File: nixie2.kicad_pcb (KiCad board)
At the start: 2 copper layers, 68.5 x 181 mm, 50 parts, among them J1 AVR-ISP-6, J14 Conn_01x10_Female, SW1 Conn_01x02_Male, SW2 Conn_01x02_Male, SW3 Conn_01x02_Male, SW4 Conn_01x02_Male, SW5 Conn_01x02_Male, SW6 Conn_01x02_Male, U1 ATmega8-16PU, U10 74141, U11 L7805, U2 74HC595, U3 74HC595, U4 74HC595, U5 74141, U6 74141, U7 74141, U8 74141, U9 74141, X1 CXO_DIP8

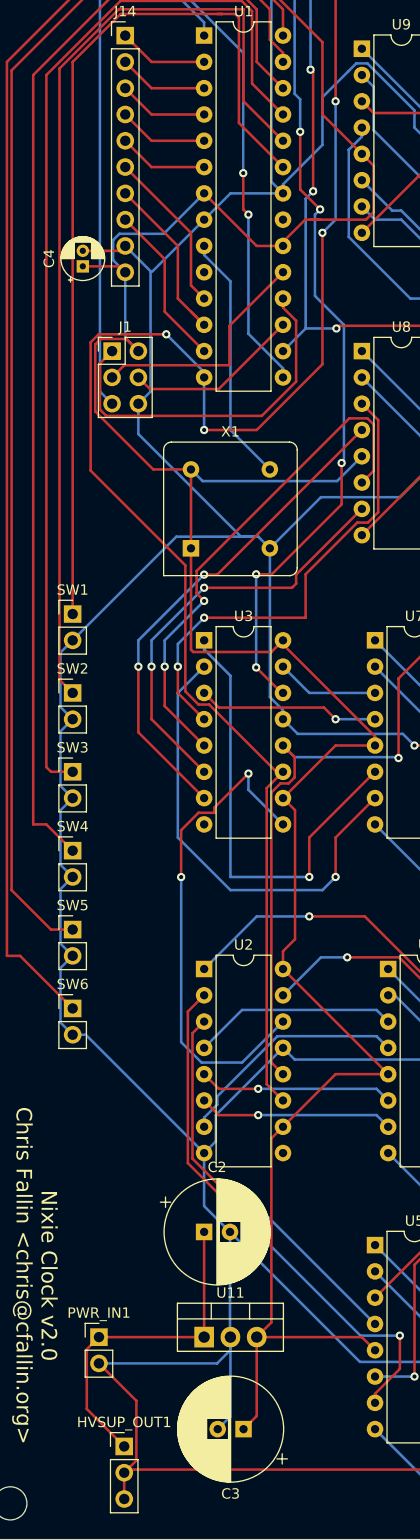
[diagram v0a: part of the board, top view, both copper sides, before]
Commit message: Update.
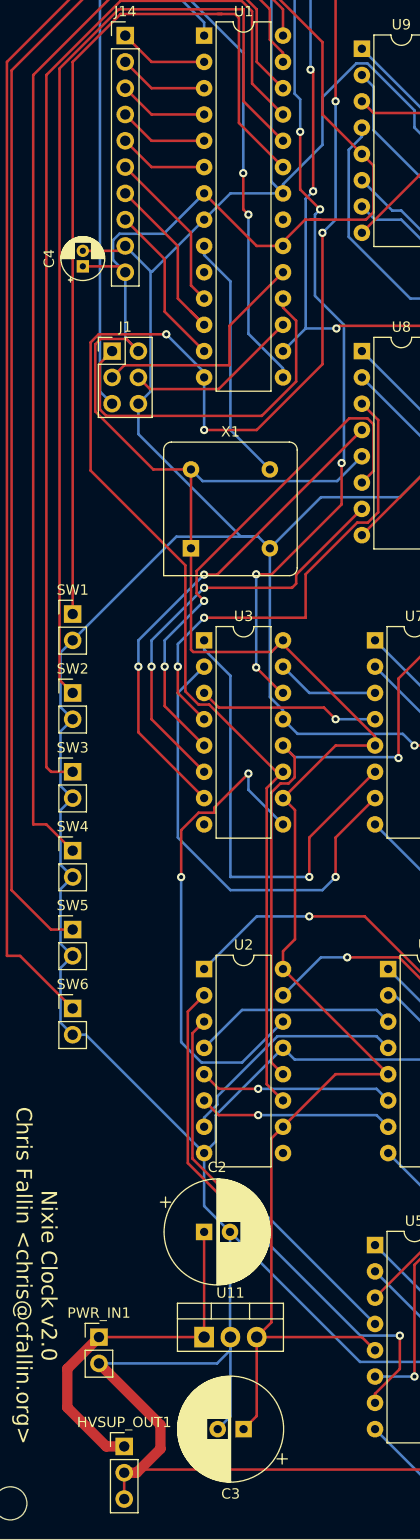
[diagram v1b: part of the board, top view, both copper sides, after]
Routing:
- net GND: track 461.4 -> 464.1 mm
- net Net-(C2-Pad1): track 32.9 -> 35.4 mm
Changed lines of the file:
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@@
     (thickness 1.6)
     (drawings 11)
-    (tracks 781)
+    (tracks 782)
     (zones 0)
     (modules 50)
@@
   )
   (setup
-    (last_trace_width 0.25)
+    (last_trace_width 1)
+    (user_trace_width 1)
     (trace_clearance 0.2)
     (zone_clearance 0.508)
@@
   (segment (start 89.734999 69.975001) (end 97.26 62.45) (width 0.25) (layer B.Cu) (net 4))
   (segment (start 89.545001 69.975001) (end 89.734999 69.975001) (width 0.25) (layer B.Cu) (net 4))
-  (segment (start 108.657499 50.657499) (end 106.15 53.164998) (width 0.25) (layer B.Cu) (net 4))
-  (segment (start 109.419999 49.894999) (end 108.657499 50.657499) (width 0.25) (layer B.Cu) (net 4))
-  (segment (start 86.63 68) (end 87.1 67.53) (width 0.25) (layer F.Cu) (net 4))
-  (segment (start 83 68) (end 86.63 68) (width 0.25) (layer F.Cu) (net 4))
-  (segment (start 88.175001 179.095001) (end 84.56 175.48) (width 0.25) (layer F.Cu) (net 4))
-  (segment (start 88.175001 184.864999) (end 88.175001 179.095001) (width 0.25) (layer F.Cu) (net 4))
-  (segment (start 87 186.04) (end 88.175001 184.864999) (width 0.25) (layer F.Cu) (net 4))
-  (segment (start 87 188.58) (end 87 186.04) (width 0.25) (layer F.Cu) (net 4))
-  (segment (start 87.305001 185.734999) (end 87 186.04) (width 0.25) (layer F.Cu) (net 4))
-  (segment (start 129.507082 185.734999) (end 87.305001 185.734999) (width 0.25) (layer F.Cu) (net 4))
+  (segment (start 109.419999 49.894999) (end 106.15 53.164998) (width 0.25) (layer B.Cu) (net 4))
+  (segment (start 86.63 68) (end 87.1 67.53) (width 0.25) (layer F.Cu) (net 4) (status 30))
+  (segment (start 83 68) (end 86.63 68) (width 0.25) (layer F.Cu) (net 4) (status 30))
+  (segment (start 87 188.58) (end 87 186.04) (width 0.25) (layer F.Cu) (net 4) (status 30))
+  (segment (start 87.305001 185.734999) (end 87 186.04) (width 0.25) (layer F.Cu) (net 4) (status 30))
+  (segment (start 129.507082 185.734999) (end 87.305001 185.734999) (width 0.25) (layer F.Cu) (net 4) (status 20))
   (segment (start 135 180.242081) (end 129.507082 185.734999) (width 0.25) (layer F.Cu) (net 4))
-  (segment (start 135 179.04) (end 135 180.242081) (width 0.25) (layer F.Cu) (net 4))
+  (segment (start 135 179.04) (end 135 180.242081) (width 0.25) (layer F.Cu) (net 4) (status 10))
+  (segment (start 88.202081 186.04) (end 90.5 183.742081) (width 1) (layer F.Cu) (net 4))
+  (segment (start 87 186.04) (end 88.202081 186.04) (width 1) (layer F.Cu) (net 4) (status 10))
+  (segment (start 90.5 181.42) (end 84.56 175.48) (width 1) (layer F.Cu) (net 4) (status 20))
+  (segment (start 90.5 183.742081) (end 90.5 181.42) (width 1) (layer F.Cu) (net 4))
   (segment (start 94.575001 90.245001) (end 93.45 89.12) (width 0.25) (layer B.Cu) (net 6) (status 20))
   (segment (start 107.564999 90.245001) (end 94.575001 90.245001) (width 0.25) (layer B.Cu) (net 6))
@@
   (segment (start 105.01 64.99) (end 110.355002 64.99) (width 0.25) (layer F.Cu) (net 6))
   (segment (start 104.484998 64.99) (end 105.01 64.99) (width 0.25) (layer F.Cu) (net 6))
-  (segment (start 86.53 69.5) (end 87.1 70.07) (width 0.25) (layer F.Cu) (net 6))
-  (segment (start 83 69.5) (end 86.53 69.5) (width 0.25) (layer F.Cu) (net 6))
+  (segment (start 86.53 69.5) (end 87.1 70.07) (width 0.25) (layer F.Cu) (net 6) (status 30))
+  (segment (start 83 69.5) (end 86.53 69.5) (width 0.25) (layer F.Cu) (net 6) (status 30))
   (segment (start 87.005001 79.054999) (end 97.165001 79.054999) (width 0.25) (layer F.Cu) (net 7))
   (segment (start 85.83 80.23) (end 87.005001 79.054999) (width 0.25) (layer F.Cu) (net 7) (status 10))
@@
   (segment (start 84.56 172.94) (end 94.72 172.94) (width 0.25) (layer F.Cu) (net 13) (status 30))
   (segment (start 94.72 172.94) (end 94.72 162.78) (width 0.25) (layer F.Cu) (net 13) (status 30))
-  (segment (start 83.384999 174.115001) (end 84.56 172.94) (width 0.25) (layer F.Cu) (net 13))
-  (segment (start 83.384999 179.884999) (end 83.384999 174.115001) (width 0.25) (layer F.Cu) (net 13))
-  (segment (start 87 183.5) (end 83.384999 179.884999) (width 0.25) (layer F.Cu) (net 13))
+  (segment (start 84.56 172.94) (end 81.5 176) (width 1) (layer F.Cu) (net 13) (status 10))
+  (segment (start 85.266 183.5) (end 87 183.5) (width 1) (layer F.Cu) (net 13) (status 20))
+  (segment (start 81.5 179.734) (end 85.266 183.5) (width 1) (layer F.Cu) (net 13))
+  (segment (start 81.5 176) (end 81.5 179.734) (width 1) (layer F.Cu) (net 13))
   (segment (start 87.1 64.99) (end 90.91 68.8) (width 0.25) (layer F.Cu) (net 14) (status 10))
   (segment (start 90.91 73.88) (end 94.72 77.69) (width 0.25) (layer F.Cu) (net 14) (status 20))
@@
   (segment (start 112.895002 64.115002) (end 109.96 61.18) (width 0.25) (layer B.Cu) (net 115) (status 20))
   (segment (start 113.77 64.115002) (end 112.895002 64.115002) (width 0.25) (layer B.Cu) (net 115))
-  (segment (start 134.5 168) (end 134.5 164) (width 0.25) (layer B.Cu) (net 116))
-  (segment (start 134 140) (end 134.5 140.5) (width 0.25) (layer B.Cu) (net 117))
-  (segment (start 134 135) (end 134 140) (width 0.25) (layer B.Cu) (net 117))
-  (segment (start 135.5 112.5) (end 135.5 105.5) (width 0.25) (layer B.Cu) (net 118))
-  (segment (start 135.5 84.5) (end 135.5 76.5) (width 0.25) (layer B.Cu) (net 119))
-  (segment (start 135 53) (end 135 47) (width 0.25) (layer B.Cu) (net 120))
-  (segment (start 135 30.5) (end 135 23) (width 0.25) (layer B.Cu) (net 121))
-  (segment (start 138.14999 58.68999) (end 135 55.54) (width 0.25) (layer B.Cu) (net 122))
+  (segment (start 134.5 168) (end 134.5 164) (width 0.25) (layer B.Cu) (net 116) (status 30))
+  (segment (start 134 140) (end 134.5 140.5) (width 0.25) (layer B.Cu) (net 117) (status 30))
+  (segment (start 134 135) (end 134 140) (width 0.25) (layer B.Cu) (net 117) (status 30))
+  (segment (start 135.5 112.5) (end 135.5 105.5) (width 0.25) (layer B.Cu) (net 118) (status 30))
+  (segment (start 135.5 84.5) (end 135.5 76.5) (width 0.25) (layer B.Cu) (net 119) (status 30))
+  (segment (start 135 53) (end 135 47) (width 0.25) (layer B.Cu) (net 120) (status 30))
+  (segment (start 135 30.5) (end 135 23) (width 0.25) (layer B.Cu) (net 121) (status 30))
+  (segment (start 138.14999 58.68999) (end 135 55.54) (width 0.25) (layer B.Cu) (net 122) (status 20))
   (segment (start 138.14999 84.39001) (end 138.14999 58.68999) (width 0.25) (layer B.Cu) (net 122))
-  (segment (start 135.5 87.04) (end 138.14999 84.39001) (width 0.25) (layer B.Cu) (net 122))
-  (segment (start 135 55.54) (end 137.5 53.04) (width 0.25) (layer B.Cu) (net 122))
-  (segment (start 137.5 35.54) (end 135 33.04) (width 0.25) (layer B.Cu) (net 122))
+  (segment (start 135.5 87.04) (end 138.14999 84.39001) (width 0.25) (layer B.Cu) (net 122) (status 10))
+  (segment (start 135 55.54) (end 137.5 53.04) (width 0.25) (layer B.Cu) (net 122) (status 10))
+  (segment (start 137.5 35.54) (end 135 33.04) (width 0.25) (layer B.Cu) (net 122) (status 20))
   (segment (start 137.5 53.04) (end 137.5 35.54) (width 0.25) (layer B.Cu) (net 122))
-  (segment (start 138.14999 112.39001) (end 135.5 115.04) (width 0.25) (layer B.Cu) (net 122))
+  (segment (start 138.14999 112.39001) (end 135.5 115.04) (width 0.25) (layer B.Cu) (net 122) (status 20))
   (segment (start 138.14999 89.68999) (end 138.14999 112.39001) (width 0.25) (layer B.Cu) (net 122))
-  (segment (start 135.5 87.04) (end 138.14999 89.68999) (width 0.25) (layer B.Cu) (net 122))
+  (segment (start 135.5 87.04) (end 138.14999 89.68999) (width 0.25) (layer B.Cu) (net 122) (status 10))
   (segment (start 138.14999 117.68999) (end 138.14999 123.85001) (width 0.25) (layer B.Cu) (net 122))
-  (segment (start 135.5 115.04) (end 138.14999 117.68999) (width 0.25) (layer B.Cu) (net 122))
+  (segment (start 135.5 115.04) (end 138.14999 117.68999) (width 0.25) (layer B.Cu) (net 122) (status 10))
   (segment (start 138.14999 123.85001) (end 138 124) (width 0.25) (layer B.Cu) (net 122))
-  (segment (start 138 139.54) (end 134.5 143.04) (width 0.25) (layer B.Cu) (net 122))
+  (segment (start 138 139.54) (end 134.5 143.04) (width 0.25) (layer B.Cu) (net 122) (status 20))
   (segment (start 138 124) (end 138 139.54) (width 0.25) (layer B.Cu) (net 122))
-  (segment (start 138.14999 166.89001) (end 134.5 170.54) (width 0.25) (layer B.Cu) (net 122))
+  (segment (start 138.14999 166.89001) (end 134.5 170.54) (width 0.25) (layer B.Cu) (net 122) (status 20))
   (segment (start 138.14999 146.68999) (end 138.14999 166.89001) (width 0.25) (layer B.Cu) (net 122))
-  (segment (start 134.5 143.04) (end 138.14999 146.68999) (width 0.25) (layer B.Cu) (net 122))
-  (segment (start 134.5 176) (end 135 176.5) (width 0.25) (layer B.Cu) (net 122))
-  (segment (start 134.5 170.54) (end 134.5 176) (width 0.25) (layer B.Cu) (net 122))
+  (segment (start 134.5 143.04) (end 138.14999 146.68999) (width 0.25) (layer B.Cu) (net 122) (status 10))
+  (segment (start 134.5 176) (end 135 176.5) (width 0.25) (layer B.Cu) (net 122) (status 30))
+  (segment (start 134.5 170.54) (end 134.5 176) (width 0.25) (layer B.Cu) (net 122) (status 30))
 )
